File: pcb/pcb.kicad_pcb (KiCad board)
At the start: 4 copper layers, 65 x 55 mm, 111 parts, among them CN1 1x4, CN10 1x2, CN11 1x2, CN12 1x8, CN2 1x8, CN3 1x8, CN4 1x8, CN5 1x4, CN6 1x2, CN7 1x2, CN8 1x8, CN9 2x5, IC1 AP2112K-3.3TRG1, IC10 SN74LVC1G17, IC11 SN74LVC1G17, IC12 SN74LVC1G17, IC13 SN74LVC1G17, IC14 SN74LVC1G17, IC15 SN74LVC1G17, IC16 SN74LVC1G17, IC17 SN74LVC1G17, IC18 SN74LVC1G17, IC19 SN74LVC1G17, IC2 STM32f103C8T, IC20 SN74LVC1G17, IC21 SN74LVC1G17, IC22 NPS4053, IC3 INA199B2, IC4 AP63301, IC5 MCP2551, IC6 SN74LVC1G17, IC7 SN74LVC1G17, IC8 SN74LVC1G17, IC9 SN74LVC1G17, SW3 219-3LPST

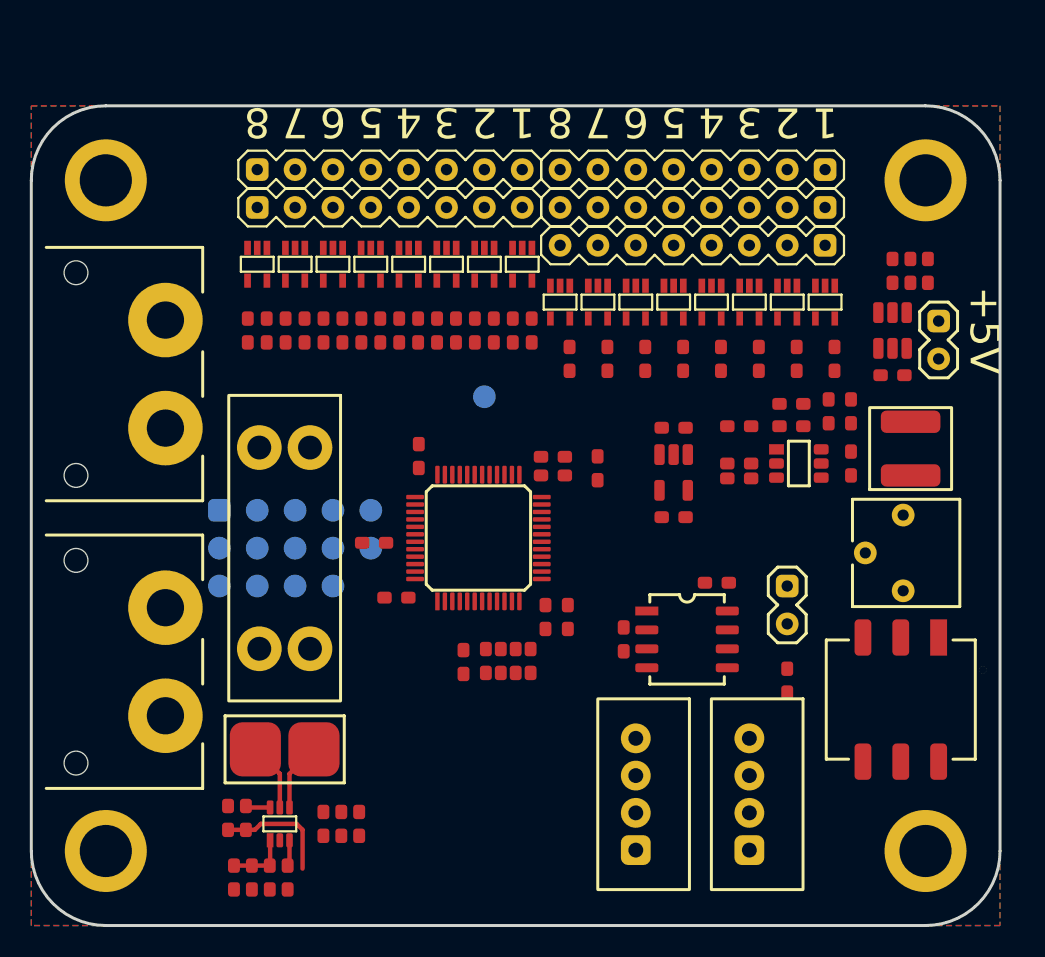
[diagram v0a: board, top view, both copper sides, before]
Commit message: worked on layout
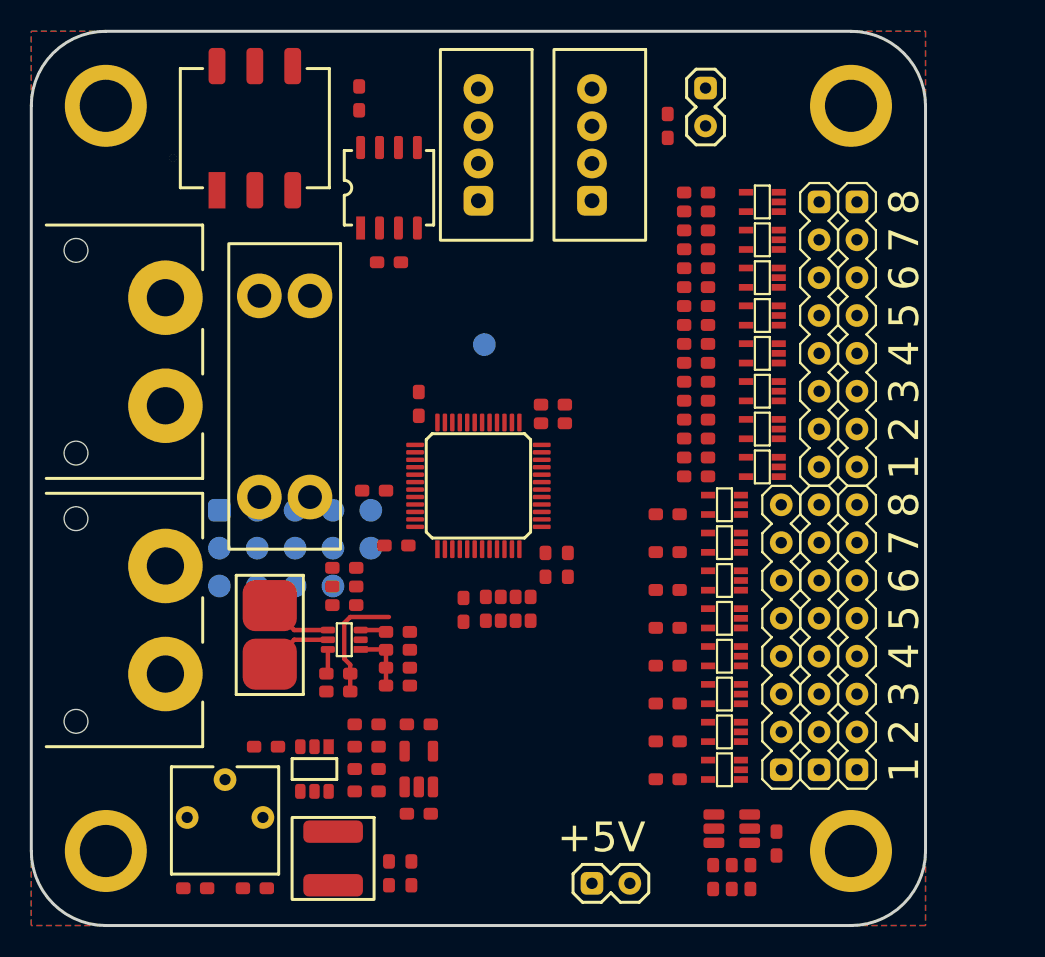
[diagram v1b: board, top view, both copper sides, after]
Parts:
- moved SW3 57.9 mm to (113.0, 77.5), turned to 90 degrees
- moved R10 48.8 mm to (111.0, 123.8), turned to 0 degrees
- moved L1 47.5 mm to (118.2, 126.5), turned to -90 degrees
- moved CN1 44.8 mm to (135.6, 78.6)
- moved CN5 44.8 mm to (128.0, 78.6)
- moved C23 43.2 mm to (113.0, 128.5), turned to 0 degrees
- moved C4 42.8 mm to (122.0, 127.5)
- moved C6 42.8 mm to (123.5, 127.5)
- moved R27 42.8 mm to (145.0, 127.8), turned to -90 degrees
- moved D2 42.1 mm to (146.2, 127.8), turned to 90 degrees
- moved CN7 40.8 mm to (138.2, 128.2), turned to 90 degrees
- moved R15 40.4 mm to (120.0, 75.5), turned to -90 degrees
- moved C21 39.2 mm to (120.5, 122.0), turned to 0 degrees
- moved R26 39.2 mm to (148.0, 125.5), turned to -90 degrees
- moved R17 39.0 mm to (109.0, 128.5), turned to 180 degrees
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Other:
- board size 65 x 55 mm -> 60 x 60 mm
- board text added: "order reversed"
- board text removed: "3.3 V"
- board text removed: "CAN bus"
- board text removed: "battery monitor"
- board text removed: "power supply"
